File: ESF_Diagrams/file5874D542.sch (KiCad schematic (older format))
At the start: 9 parts

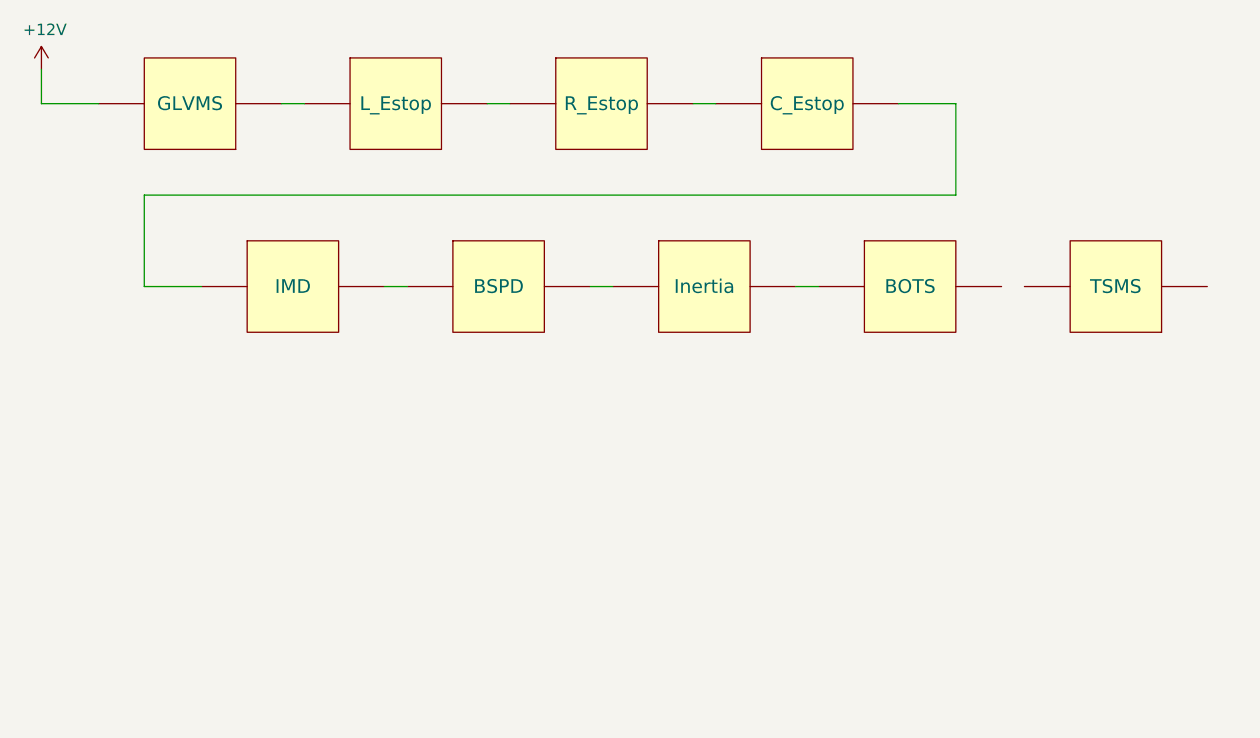
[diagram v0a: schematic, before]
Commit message: ESF Fixes
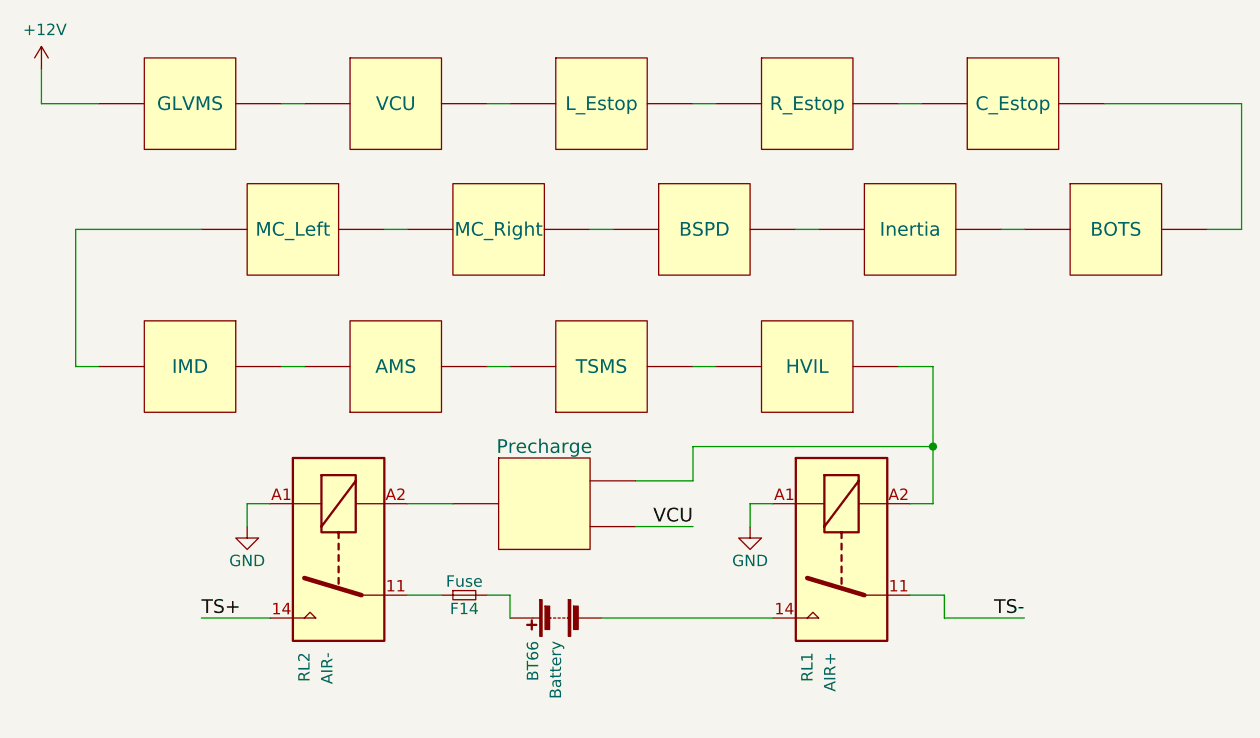
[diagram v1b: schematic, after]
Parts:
- added BT66: Battery, symbol Battery
- added F14: Fuse, symbol Fuse_Small
- added RL1: AIR+, symbol Relay-SPST
- added RL2: AIR-, symbol Relay-SPST
- added U13: MC_Left, symbol Generic_1x1
- added U15: VCU, symbol Generic_1x1
- added U16: MC_Right, symbol Generic_1x1
- added U19: HVIL, symbol Generic_1x1
- added U25: AMS, symbol Generic_1x1
- added U26: Precharge, symbol Generic_1x2
- gave numbers to parts that had none: 9
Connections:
- net at U17.~: now also U25.~; no longer U20.~
- net at U23.~: now also U24.~; no longer U17.~
- net at U20.~: now also U16.~; no longer U22.~
- net at U18.~: now also U15.~; no longer U12.~
- net at U14.~: now also U25.~
- net at U21.~: now also U23.~; no longer U18.~
- new net: U13.~, U17.~
- new net: U20.~, U22.~
- new net: U12.~, U15.~
- new net: U14.~, U19.~
- new net: U18.~, U21.~
- new net: U13.~, U16.~
- new net: BT66.2 (-), RL1.14
- new net: RL1.A2, U19.~, U26.~
- new net: F14.1, RL2.11
- new net: RL2.A2, U26.~
- new net: BT66.1 (+), F14.2
- new net GND: RL1.A1, RL2.A1
- new net TS+: RL2.14
- new net TS-: RL1.11
- new net VCU: U26.~
